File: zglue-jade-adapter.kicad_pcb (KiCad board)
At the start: 6 copper layers, 25 x 20 mm, 77 parts, among them J1 543630489, J2 543630489, U1 zGlue-Jade

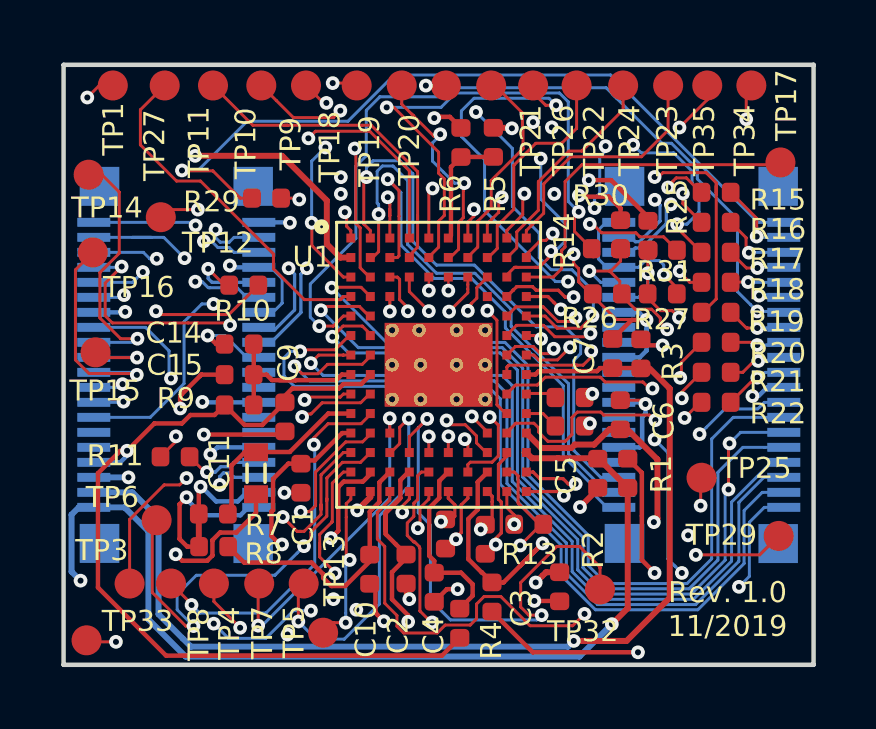
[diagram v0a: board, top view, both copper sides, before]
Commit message: Regenerate libraries
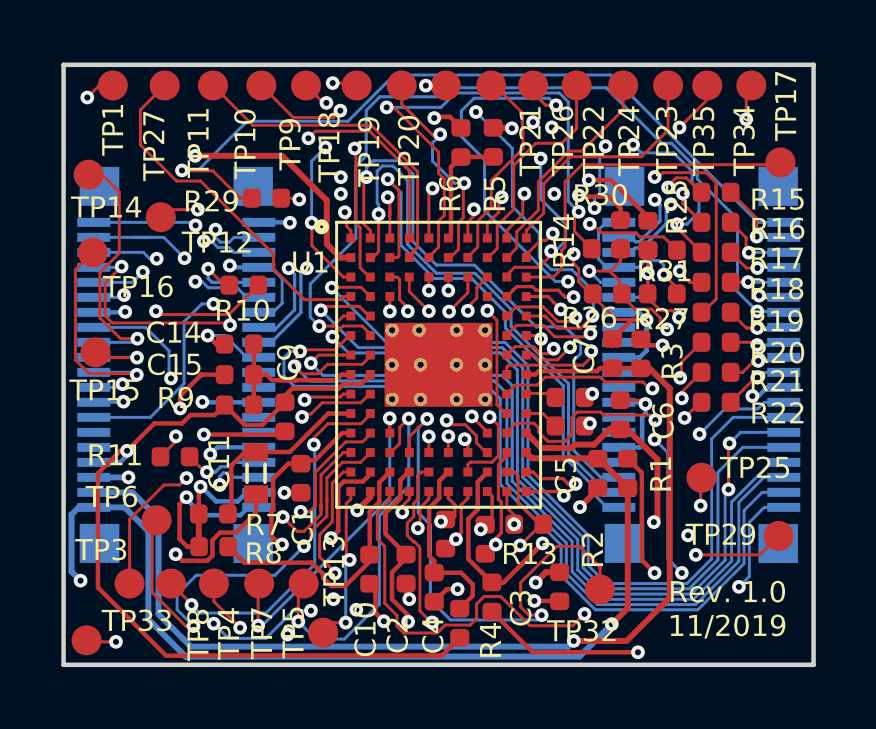
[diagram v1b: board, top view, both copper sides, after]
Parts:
- C1, C10, C14, C15, C2, C3, C4, C5, C6, C7, C9: footprint antmicro-footprints:0402-cap -> zglue-jade-adapter-footprints:0402-cap
- C11: footprint antmicro-footprints:0603-cap -> zglue-jade-adapter-footprints:0603-cap
- J1, J2: footprint antmicro-footprints:543630489 -> zglue-jade-adapter-footprints:543630489
- R1, R10, R11, R12, R13, R14, R15, R16, R17, R18, R19, R2, R20, R21, R22, R23, R24, R25, R26, R27, R28, R29, R3, R30, R31, R4, R5, R6, R7, R8, R9: footprint antmicro-footprints:0402-res -> zglue-jade-adapter-footprints:0402-res
- TP1, TP10, TP11, TP12, TP13, TP14, TP15, TP16, TP17, TP18, TP19, TP20, TP21, TP22, TP23, TP24, TP25, TP26, TP27, TP29, TP3, TP32, TP33, TP34, TP35, TP4, TP5, TP6, TP7, TP8, TP9: footprint antmicro-footprints:Testpoint_smd_1mm -> zglue-jade-adapter-footprints:Testpoint_smd_1mm
- U1: footprint lib:Z-Glue_LGA-96 -> zglue-jade-adapter-footprints:Z-Glue_LGA-96
